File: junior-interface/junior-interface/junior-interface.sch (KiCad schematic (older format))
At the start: 19 parts, among them IC13 7427, IC14 74LS01, IC15 74LS30, IC16 74LS00, IC17 GAL16V8, IC2 2114, IC3 2114, IC4 2716, IC5 2716, J12 Conn_01x03_Male

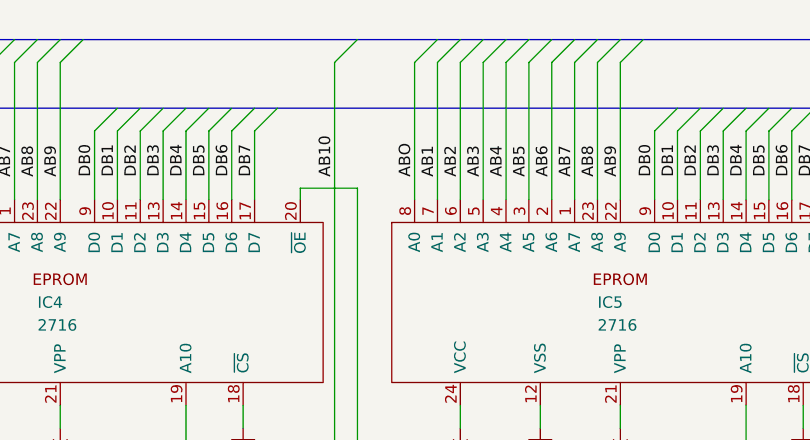
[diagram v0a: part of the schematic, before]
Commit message: junior interface routage
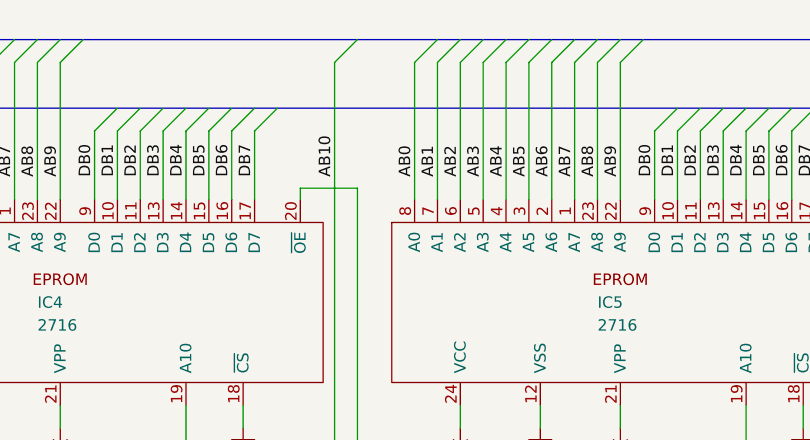
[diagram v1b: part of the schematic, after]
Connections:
- net ABO is gone; now on net AB0: IC5.8 (A0)
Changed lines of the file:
@@
 DB7
 Text Label 3450 1450 1    50   ~ 0
-ABO
+AB0
 Text Label 3100 1450 1    50   ~ 0
 AB10

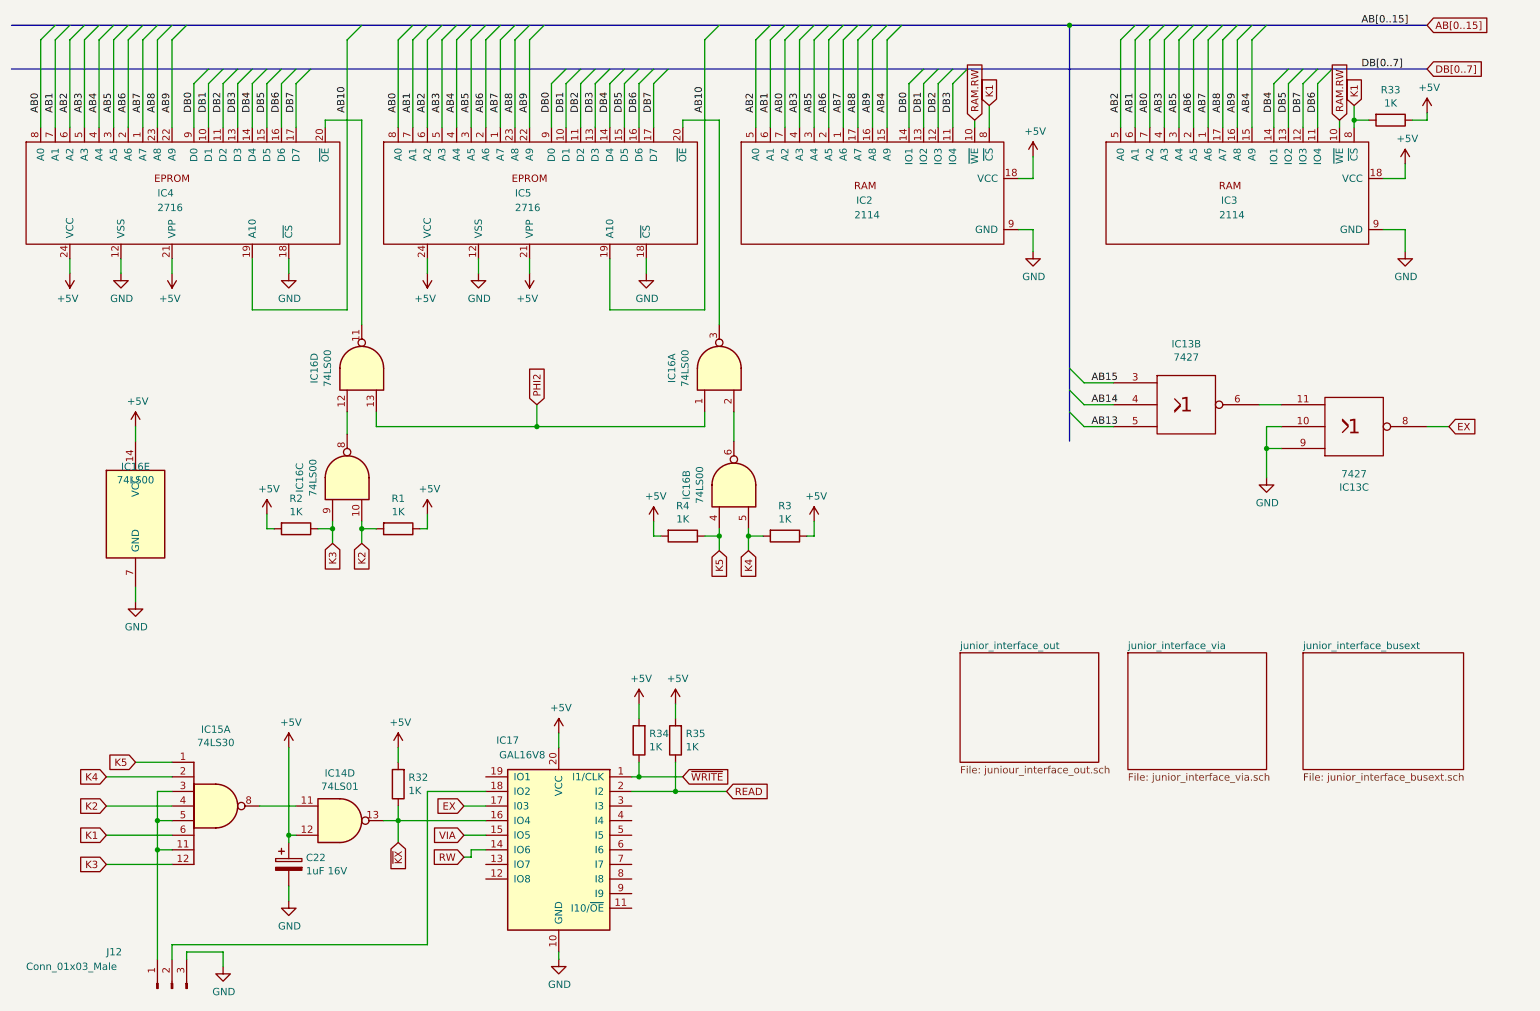
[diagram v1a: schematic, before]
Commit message: junior interface routage
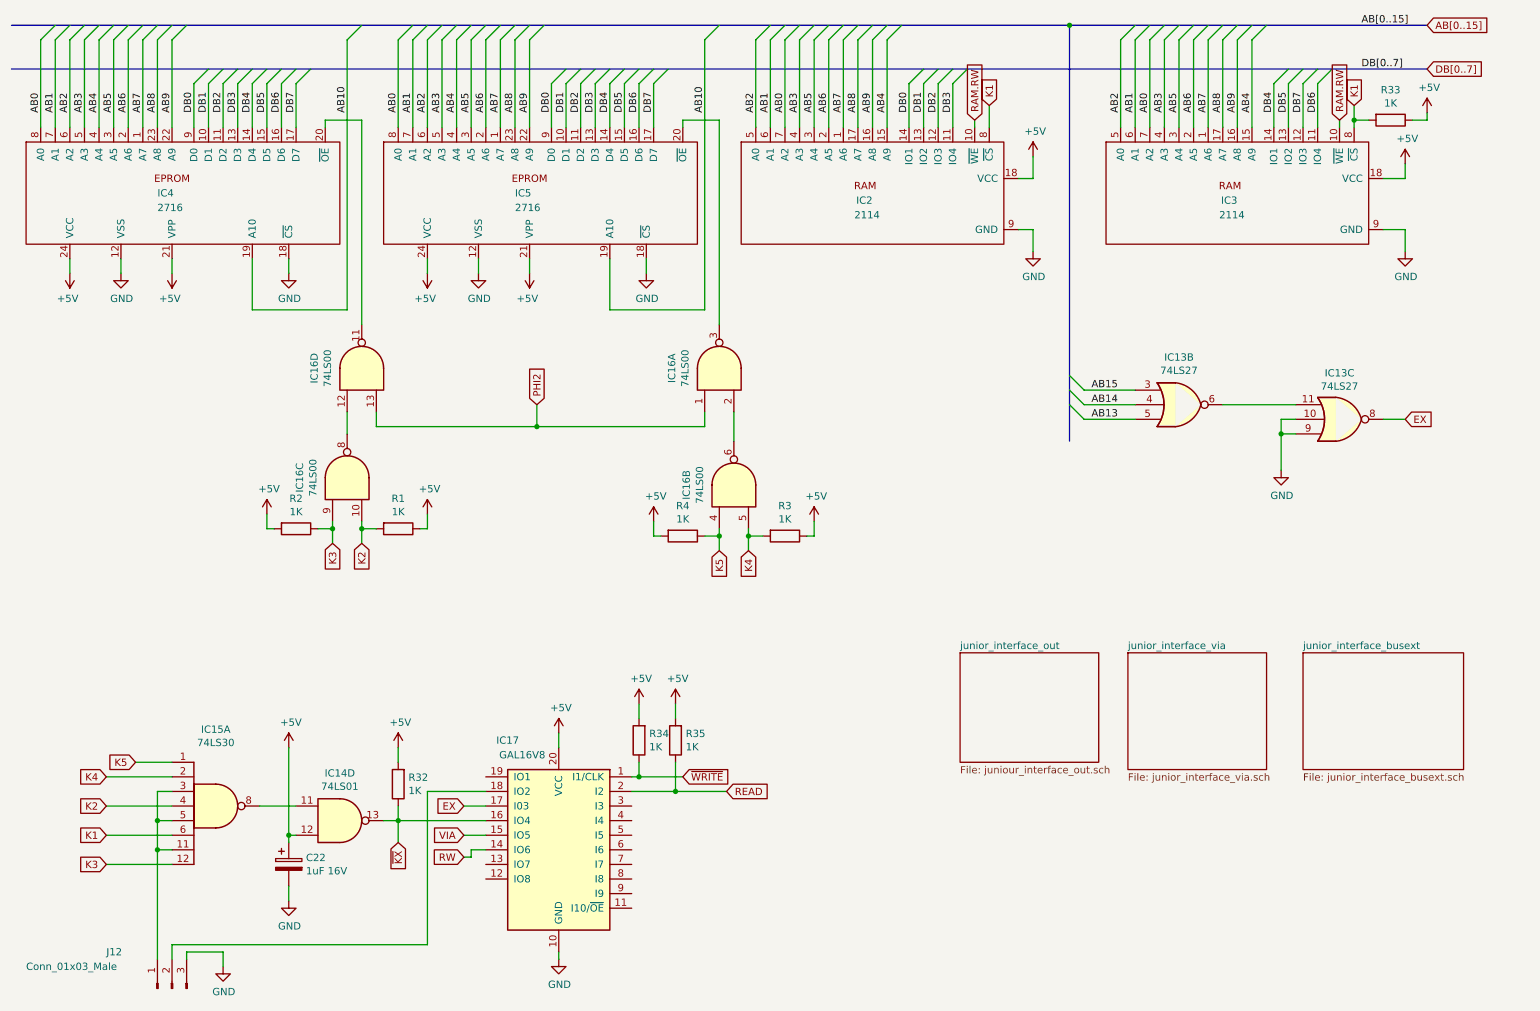
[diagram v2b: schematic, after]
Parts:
- removed IC13: 7427, elektor:DIL-14, symbol 74xx_IEEE:7427
- removed unit 5 of IC16
- added IC13: 74LS27, symbol 74xx:74LS27
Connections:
- net AB13: now also IC13.5
- net AB14: now also IC13.4
- net AB15: now also IC13.3
- net EX: now also IC13.8
- net GND: now also IC13.10, IC13.9
- new net: IC13.11, IC13.6
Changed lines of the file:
@@
-$EndComp
-$Comp
-L 74xx_IEEE:7427 IC13
-U 2 1 5F9376A0
-P 8850 3450
-F 0 "IC13" H 8850 3866 50  0000 C CNN
-F 1 "7427" H 8850 3775 50  0000 C CNN
-F 2 "elektor:DIL-14" H 8850 3450 50  0001 C CNN
-F 3 "" H 8850 3450 50  0001 C CNN
-	2    8850 3450
-	1    0    0    -1
 $EndComp
 $Comp
@@
 	2550 4300 2600 4300
 $Comp
-L 74xx:74LS00 IC16
-U 5 1 5FBBFF19
-P 1650 4200
-F 0 "IC16" H 1650 4525 50  0000 C CNN
-F 1 "74LS00" H 1650 4434 50  0000 C CNN
-F 2 "elektor:DIL-14" H 1650 4200 50  0001 C CNN
-F 3 "http://www.ti.com/lit/gpn/sn74ls00" H 1650 4200 50  0001 C CNN
-	5    1650 4200
-	1    0    0    -1
-$EndComp
-$Comp
-L power:+5V #PWR0130
-U 1 1 5FBCAC8D
-P 1650 3600
-F 0 "#PWR0130" H 1650 3450 50  0001 C CNN
-F 1 "+5V" H 1665 3773 50  0000 C CNN
-F 2 "" H 1650 3600 50  0001 C CNN
-F 3 "" H 1650 3600 50  0001 C CNN
-	1    1650 3600
-	1    0    0    -1
-$EndComp
-$Comp
-L power:GND #PWR0131
-U 1 1 5FBCAF08
-P 1650 4800
-F 0 "#PWR0131" H 1650 4550 50  0001 C CNN
-F 1 "GND" H 1655 4627 50  0000 C CNN
-F 2 "" H 1650 4800 50  0001 C CNN
-F 3 "" H 1650 4800 50  0001 C CNN
-	1    1650 4800
-	1    0    0    -1
-$EndComp
-Wire Wire Line
-	1650 3600 1650 3700
-Wire Wire Line
-	1650 4700 1650 4800
-$Comp
-L 74xx_IEEE:7427 IC13
-U 3 1 5FBDF24B
-P 10000 3600
-F 0 "IC13" H 10000 4016 50  0000 C CNN
-F 1 "7427" H 10000 3925 50  0000 C CNN
-F 2 "elektor:DIL-14" H 10000 3600 50  0001 C CNN
-F 3 "" H 10000 3600 50  0001 C CNN
-	3    10000 3600
-	1    0    0    1
-$EndComp
-$Comp
 L power:GND #PWR0132
 U 1 1 5FBDF64E
-P 9400 3950
-F 0 "#PWR0132" H 9400 3700 50  0001 C CNN
-F 1 "GND" H 9405 3777 50  0000 C CNN
-F 2 "" H 9400 3950 50  0001 C CNN
-F 3 "" H 9400 3950 50  0001 C CNN
-	1    9400 3950
-	1    0    0    -1
-$EndComp
-Wire Wire Line
-	9500 3600 9400 3600
-Wire Wire Line
-	9400 3600 9400 3750
-Wire Wire Line
-	9500 3750 9400 3750
-Connection ~ 9400 3750
-Wire Wire Line
-	9400 3750 9400 3950
-Wire Wire Line
-	9350 3450 9500 3450
+P 9500 3900
+F 0 "#PWR0132" H 9500 3650 50  0001 C CNN
+F 1 "GND" H 9505 3727 50  0000 C CNN
+F 2 "" H 9500 3900 50  0001 C CNN
+F 3 "" H 9500 3900 50  0001 C CNN
+	1    9500 3900
+	1    0    0    -1
+$EndComp
+Wire Wire Line
+	9600 3550 9500 3550
+Wire Wire Line
+	9500 3550 9500 3650
 Connection ~ 8050 850
 Entry Wire Line
-	8050 3200 8150 3300
+	8050 3250 8150 3350
 Entry Wire Line
 	8050 3350 8150 3450
 Entry Wire Line
-	8050 3500 8150 3600
-Wire Wire Line
-	8350 3300 8150 3300
-Wire Wire Line
-	8150 3450 8350 3450
-Wire Wire Line
-	8150 3600 8350 3600
-Text Label 8200 3300 0    50   ~ 0
+	8050 3450 8150 3550
+Text Label 8200 3350 0    50   ~ 0
 AB15
 Text Label 8200 3450 0    50   ~ 0
 AB14
-Text Label 8200 3600 0    50   ~ 0
+Text Label 8200 3550 0    50   ~ 0
 AB13
-Text GLabel 10650 3600 2    50   Input ~ 0
+Text GLabel 10350 3550 2    50   Input ~ 0
 EX
 Wire Wire Line
-	10650 3600 10500 3600
+	10350 3550 10200 3550
 Text GLabel 1650 5900 0    50   Input ~ 0
 K5
@@
 Text Label 10050 1150 0    50   ~ 0
 DB[0..7]
+$Comp
+L 74xx:74LS27 IC13
+U 2 1 5F9B8CFD
+P 8800 3450
+F 0 "IC13" H 8800 3775 50  0000 C CNN
+F 1 "74LS27" H 8800 3684 50  0000 C CNN
+F 2 "" H 8800 3450 50  0001 C CNN
+F 3 "http://www.ti.com/lit/gpn/sn74LS27" H 8800 3450 50  0001 C CNN
+	2    8800 3450
+	1    0    0    -1
+$EndComp
+Wire Wire Line
+	8150 3350 8500 3350
+Wire Wire Line
+	8150 3450 8500 3450
+Wire Wire Line
+	8150 3550 8500 3550
+$Comp
+L 74xx:74LS27 IC13
+U 3 1 5F9DFDD4
+P 9900 3550
+F 0 "IC13" H 9900 3233 50  0000 C CNN
+F 1 "74LS27" H 9900 3324 50  0000 C CNN
+F 2 "" H 9900 3550 50  0001 C CNN
+F 3 "http://www.ti.com/lit/gpn/sn74LS27" H 9900 3550 50  0001 C CNN
+	3    9900 3550
+	1    0    0    1
+$EndComp
+Wire Wire Line
+	9600 3650 9500 3650
+Connection ~ 9500 3650
+Wire Wire Line
+	9500 3650 9500 3900
+Wire Wire Line
+	9100 3450 9600 3450
 Wire Bus Line
 	8050 850  8050 3700
